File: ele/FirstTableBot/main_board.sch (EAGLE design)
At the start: 2 parts

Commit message: Vzber sensoru
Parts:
- removed JP1: PINH2X06, pinhead_smd:PINH2X06
- added JP2: PINH2X08, pinhead_smd:PINH2X08
- added R1, R10, R11, R12, R13, R14, R2, R3, R4, R5, R6, R7, R8, R9: (no value), resistor:R-EU_R0603
- added U$1, U$2, U$3, U$4, U$5, U$6, U$7: CNY70, cny70:CNY70
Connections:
- new net ADC0: MLF1.PA3/ADC0/T1/SNS, R2.1, U$2.COL
- new net ADC1: MLF1.PA4/ADC1/T0, R4.1, U$1.COL
- new net ADC11: MLF1.ADC11/CLK0/PC2
- new net ADC2: MLF1.PA5/ADC2/OC0B, R6.1, U$3.COL
- new net ADC3: MLF1.PA6/ADC3/OC1B, R8.1, U$4.COL
- new net ADC4: MLF1.PA7/RXD0/ADC4, R10.1, U$5.COL
- new net ADC5: MLF1.PB0/TXD0/ADC5, R12.1, U$6.COL
- new net ADC6: R14.1, U$7.COL
- new net ADC8: MLF1.ADC8/OC1A/PB3
- new net ADC9: MLF1.ADC9/OC0A/XCK0/PC0
- new net N$1: R1.2, U$2.A
- new net N$2: R3.2, U$1.A
- new net N$3: R5.2, U$3.A
- new net N$4: R7.2, U$4.A
- new net N$5: R9.2, U$5.A
- new net N$6: R11.2, U$6.A
- new net N$7: R13.2, U$7.A
- new net SCK: JP2B6.1, JP2T6.1
- net +5V: now also JP2B2.1, JP2T2.1, R1.1, R10.2, R11.1, R12.2, R13.1, R14.2, R2.2, R3.1, R4.2, R5.1, R6.2, R7.1, R8.2, R9.1; no longer JP1B1.1, JP1T1.1
- net CLK: now also JP2B5.1, JP2T5.1; no longer JP1B4.1, JP1T4.1
- net GND: now also JP2B3.1, JP2B4.1, JP2T3.1, JP2T4.1, U$1.C, U$1.EMI, U$2.C, U$2.EMI, U$3.C, U$3.EMI, U$4.C, U$4.EMI, U$5.C, U$5.EMI, U$6.C, U$6.EMI, U$7.C, U$7.EMI; no longer JP1B6.1, JP1T6.1
- net MISO: now also JP2B7.1, JP2T7.1; no longer JP1B3.1, JP1T3.1
- net MOSI: now also JP2B8.1, JP2T8.1; no longer JP1B2.1, JP1T2.1
- net RESET: now also JP2B1.1, JP2T1.1; no longer JP1B5.1, JP1T5.1

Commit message: schem
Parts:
- added C1, C2: 10u, rcl_upravena:C-EUC1206
- added C3, C4, C5, C8, C9: 100n, rcl_upravena:C-EUC1206
- added C6, C7: (no value), rcl:CPOL-EUE5-10.5
- added D2: (no value), diode:DIODE-D-7.5
- added D3: (no value), diode:SCHOTTKY-DIODEF126Z12
- added IM10: DRV8833_BOARD, DRV8833board:DRV8833_BOARD
- added IM6: DEVKITC, esp32:DEVKITC
- added JP3, JP5, JP6: (no value), pinhead:PINHD-1X3
- added JP30: IM10_ULT, pinhead:PINHD-1X1
- added JP4: (no value), pinhead:PINHD-2X5
- added LED0, LED1, LED2, LED3, LED5: BLUE, led:LED3MM
- added LED4: RED, led:LED3MM
- added NC1, NC2, NC3, NC4, NC5, NC6: NC, NC:NC
- added Q2, Q5: (no value), transistors:P-MOSFET-TO220V
- added Q3: (no value), transistors:N-MOSFET-SOT23-DIST
- added Q6: (no value), transistors:N-MOSFET-SOT23-GSD
- added R15: 2M, rcl_upravena:R-EU_R0805
- added R16, R19: 10k, rcl_upravena:R-EU_R0805
- added R17: 100k, rcl_upravena:R-EU_R0805
- added R18: 2M, rcl_upravena:R-EU_M0805
- added R20: (no value), pot:TRIM_US-SM-42/43X
- added R21, R22: 5k, resistor:R-EU_R0402
- added R24: (no value), resistor:R-EU_R0603
- added RN1: (no value), resistor-dil:2R-NEXB24V
- added RN2: (no value), resistor-dil:4R-N0402ARV341
- added SW0, SW1, SW2, SW3, SW4, SW5, SW6: (no value), switch-omron:10-XX
- added X1, X2: M8, con-wago-508:W237-02P
- added X4: POWER_IN, con-wago-508:W237-02P
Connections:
- new net +3V3: IM6.3V3, Q3.G, R16.1, R19.2, R22.1
- new net +5V_ESP: D2.C, IM6.5V
- new net BAT1: Q5.D, X4-2.KL
- new net BAT_POL+: Q2.S, Q5.S, R17.1, R24.2
- new net EN: IM6.EN, R19.1
- new net GPIO0: IM6.IO0
- new net GPIO12: IM6.IO12
- new net GPIO14: IM6.IO14
- new net GPIO15: IM6.IO15
- new net GPIO16: IM6.IO16, JP5.1
- new net GPIO17: IM6.IO17, JP3.1
- new net GPIO18: IM6.IO18
- new net GPIO19: IM6.IO19
- new net GPIO2: IM6.IO2
- new net GPIO21: IM6.IO21, Q3.S, R22.2
- new net GPIO22: IM6.IO22
- new net GPIO23: IM6.IO23
- new net GPIO25: IM6.IO25
- new net GPIO26: IM6.IO26
- new net GPIO27: IM6.IO27
- new net GPIO32: IM6.IO32
- new net GPIO33: IM6.IO33, R20.S
- new net GPIO34: IM6.IO34
- new net GPIO35: IM6.IO35
- new net GPIO36: IM6.SVP
- new net GPIO39: IM6.SVN
- new net GPIO4: IM6.IO4
- new net GPIO5: IM6.IO5
- new net IO1: IM6.TXD0
- new net IO10_NC: IM6.SD3, NC2.NC
- new net IO10_NC1: IM6.SD0, NC5.NC
- new net IO11_NC: IM6.CMD, NC3.NC
- new net IO11_NC1: IM6.SD1, NC6.NC
- new net IO3: IM6.RXD0
- new net IO9_NC: IM6.SD2, NC1.NC
- new net IO9_NC1: IM6.CLK, NC4.NC
- new net M1A: IM10.OUT1, X1-1.KL
- new net M1B: IM10.OUT2, X1-2.KL
- new net M2A: IM10.OUT3, X2-1.KL
- new net M2B: IM10.OUT4, X2-2.KL
- new net N$10: LED5.A, R24.1
- new net N$11: JP6.1, Q3.D, R21.1
- new net N$8: IM10.ULT, JP30.1
- new net N$9: C2.1, Q6.G, R15.1, R16.2, SW5.P, SW5.P1
- new net OFF: IM6.IO13
- new net PA0: MLF1.PA0/AREF, RN2A.1
- new net PA1: MLF1.PA1/AIN0, RN2B.1
- new net PA2: MLF1.PA2/AIN1, RN2C.1
- new net PC4: MLF1.XTAL2/PC4, RN2D.1
- new net PC5: MLF1.XTAL1/PC5, RN1A.1
- new net PWM0: IM10.IN1
- new net PWM1: IM10.IN2
- new net PWM2: IM10.IN3
- new net PWM3: IM10.IN4
- new net SLEEP: IM10.!SLEEP
- new net START_GATE1: C1.1, Q2.G, Q6.D, R17.2, R18.1
- new net SW0: C5.2, JP4.10, LED3.A, RN2A.2, SW0.P, SW0.P1
- new net SW1: C3.2, JP4.8, LED2.A, RN2B.2, SW1.P, SW1.P1
- new net SW2: C4.2, JP4.6, LED1.A, RN2C.2, SW2.P, SW2.P1
- new net SW3: C8.2, JP4.4, LED0.A, RN2D.2, SW3.P, SW3.P1
- new net SW4: C9.2, JP4.2, LED4.A, RN1A.2, SW6.P, SW6.P1
- new net VCC: C6.+, C7.+, D3.C, IM10.VCC, JP3.2, JP5.2, Q2.D, R20.A
- net +5V: now also D2.A, JP6.2, R21.2
- net GND: now also C1.2, C2.2, C3.1, C4.1, C5.1, C6.-, C7.-, C8.1, C9.1, D3.A, IM10.GND, IM6.GND, JP3.3, JP4.1, JP4.3, JP4.5, JP4.7, JP4.9, JP5.3, JP6.3, LED0.C, LED1.C, LED2.C, LED3.C, LED4.C, LED5.C, Q5.G, Q6.S, R15.2, R18.2, R20.E, SW0.S, SW0.S1, SW1.S, SW1.S1, SW2.S, SW2.S1, SW3.S, SW3.S1, SW4.P, SW4.P1, SW4.S, SW4.S1, SW5.S, SW5.S1, SW6.S, SW6.S1, X4-1.KL
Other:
- note added: "delic na mereni baterek"
- note added: "inteligentní ledky"
- note added: "rezerve_ADC1"

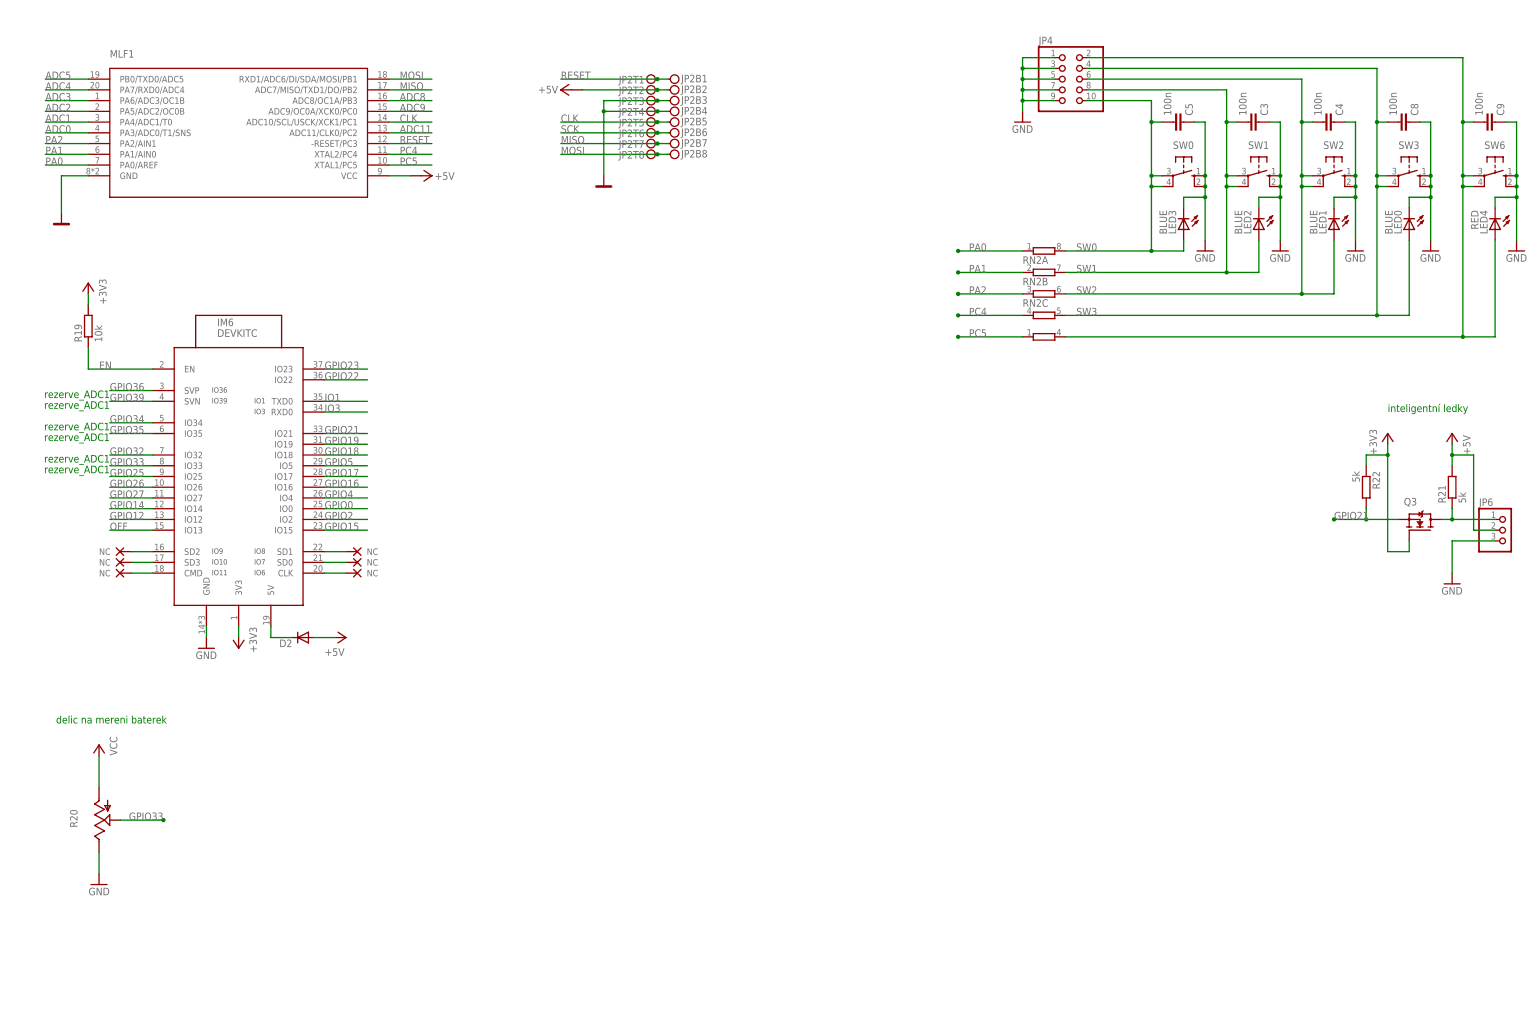
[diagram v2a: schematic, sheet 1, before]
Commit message: zmena ATtiny
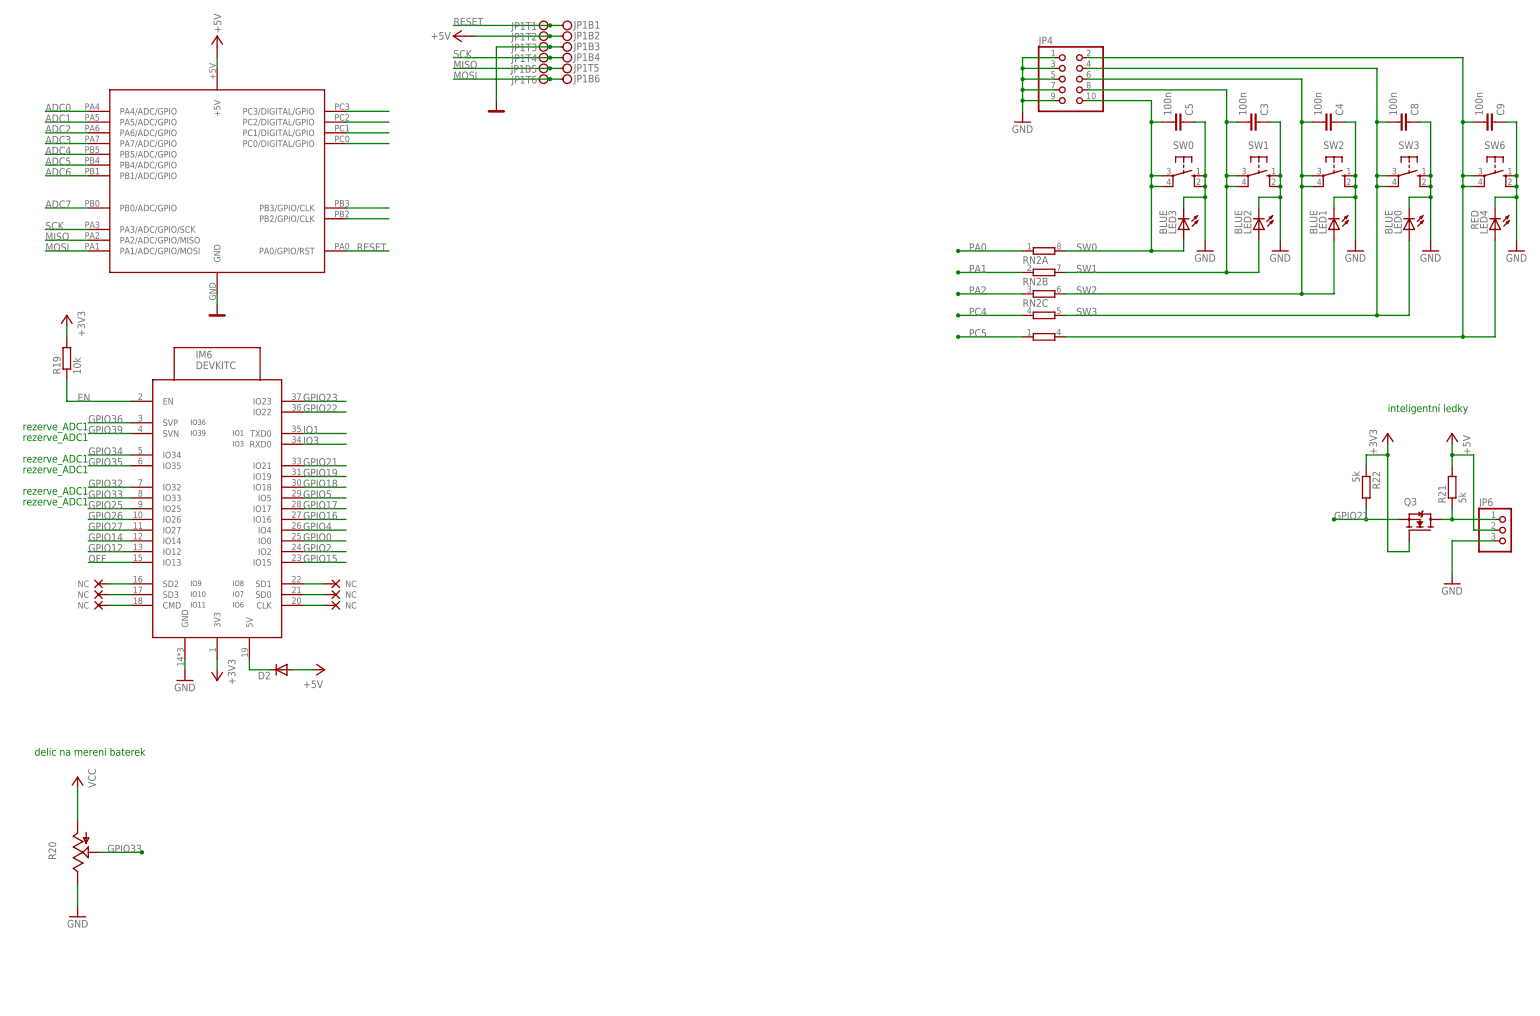
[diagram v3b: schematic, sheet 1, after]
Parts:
- removed JP2: PINH2X08, pinhead_smd:PINH2X08
- removed MLF1: ATTINY1634MLF20, attiny1634:ATTINY1634MLF20
- added JP1: PINH2X06, pinhead_smd:PINH2X06
- added U$8: ATTINI1616SOIC, ATTINY1616:ATTINI1616SOIC
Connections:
- removed net ADC11: MLF1.ADC11/CLK0/PC2
- removed net ADC8: MLF1.ADC8/OC1A/PB3
- removed net ADC9: MLF1.ADC9/OC0A/XCK0/PC0
- removed net CLK: JP2B5.1, JP2T5.1, MLF1.ADC10/SCL/USCK/XCK1/PC1
- new net ADC7: U$8.PB0/ADC/GPIO
- new net N$24: U$8.PB2/GPIO/CLK
- new net N$25: U$8.PB3/GPIO/CLK
- new net N$26: U$8.PC0/DIGITAL/GPIO
- new net N$27: U$8.PC1/DIGITAL/GPIO
- new net N$28: U$8.PC2/DIGITAL/GPIO
- new net N$29: U$8.PC3/DIGITAL/GPIO
- net +5V: now also JP1B2.1, JP1T2.1, U$8.+5V; no longer JP2B2.1, JP2T2.1, MLF1.VCC
- net ADC0: now also U$8.PA4/ADC/GPIO; no longer MLF1.PA3/ADC0/T1/SNS
- net ADC1: now also U$8.PA5/ADC/GPIO; no longer MLF1.PA4/ADC1/T0
- net ADC2: now also U$8.PA6/ADC/GPIO; no longer MLF1.PA5/ADC2/OC0B
- net ADC3: now also U$8.PA7/ADC/GPIO; no longer MLF1.PA6/ADC3/OC1B
- net ADC4: now also U$8.PB5/ADC/GPIO; no longer MLF1.PA7/RXD0/ADC4
- net ADC5: now also U$8.PB4/ADC/GPIO; no longer MLF1.PB0/TXD0/ADC5
- net ADC6: now also U$8.PB1/ADC/GPIO
- net GND: now also JP1B3.1, JP1T3.1, U$8.GND; no longer JP2B3.1, JP2B4.1, JP2T3.1, JP2T4.1, MLF1.GND
- net MISO: now also JP1B5.1, JP1T5.1, U$8.PA2/ADC/GPIO/MISO; no longer JP2B7.1, JP2T7.1, MLF1.ADC7/MISO/TXD1/DO/PB2
- net MOSI: now also JP1B6.1, JP1T6.1, U$8.PA1/ADC/GPIO/MOSI; no longer JP2B8.1, JP2T8.1, MLF1.RXD1/ADC6/DI/SDA/MOSI/PB1
- net PA0: no longer MLF1.PA0/AREF
- net PA1: no longer MLF1.PA1/AIN0
- net PA2: no longer MLF1.PA2/AIN1
- net PC4: no longer MLF1.XTAL2/PC4
- net PC5: no longer MLF1.XTAL1/PC5
- net RESET: now also JP1B1.1, JP1T1.1, U$8.PA0/GPIO/RST; no longer JP2B1.1, JP2T1.1, MLF1.-RESET/PC3
- net SCK: now also JP1B4.1, JP1T4.1, U$8.PA3/ADC/GPIO/SCK; no longer JP2B6.1, JP2T6.1
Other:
- moved on the sheet: D2, IM6, R19, R20

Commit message: DRV8833_jen_svab
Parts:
- removed D2: (no value), diode:DIODE-D-7.5
- removed IM10: DRV8833_BOARD, DRV8833board:DRV8833_BOARD
- removed IM6: DEVKITC, esp32:DEVKITC
- removed JP30: IM10_ULT, pinhead:PINHD-1X1
- removed NC2, NC3, NC4, NC5, NC6: NC, NC:NC
- removed R19: 10k, rcl_upravena:R-EU_R0805
- removed X1, X2: M8, con-wago-508:W237-02P
- added !CTS, !DCD, !DSR, !DTR, !RESET, !RTS, !SUSPEND, CHR0, CHR1, CHREN, IO0/TXLED, IO1/RXLED, IO2/RS485, IO3/WAKEUP, IO4, IO5, IO6, RI/CLK, RXD, SUSPEND, TXD: PINH1X01, pinhead_smd:PINH1X01
- added B1, B2: TACTM-35N-F, TACTM-35N-F:TACTM-35N-F
- added C10, C14, C19, C22: 100n/16V, rcl_upravena:C-EUC0402
- added C11, C12, C13, C18: 4u7/16V, rcl_upravena:C-EUC0603
- added C23: 100nf, resistor:C-EUC0603
- added C37: 330u/16V, rcl_upravena:CPOL-EUE5-10.5
- added D1, D4: skl34, diode:SHOTTKY-SOD123
- added EN, JP36, JP38, VUSB: (no value), pinhead:PINHD-1X2
- added IC3: CP2102N-28, CP2102N:CP2102N-28
- added IM3: STEPDOWN, StepDown:STEPDOWN
- added JP11: (no value), pinhead:PINHD-1X8
- added JP2, PWR_1: (no value), pinhead:PINHD-2X12
- added JP7, PWR_2: (no value), pinhead:PINHD-2X14
- added LED6, LED7, LED8: yellow, led:LEDCHIP-LED0603
- added LED_3V3: green, led:LEDCHIPLED_0603
- added NC7: NC, NC:NC
- added R23, R25, R26, R31: 470R, rcl_upravena:R-EU_R0603
- added R27, R28, R58, R60, R61: 10k, rcl_upravena:R-EU_R0603
- added R29, R30, R32, R33, R34, R35, R36, R37, R38, R39, R40, R41, R42, R43, R44, R45, R46, R47, R48, R49, R50, R51, R52, R53, R54, R55, R56, R57: 180R, rcl_upravena:R-EU_R0603
- added R59: 100k, rcl_upravena:R-EU_R0603
- added T1, T2: BC337, transistors:NPN-SOT23-BEC
- added U$9: DRV8833HTSSOP, texas-cc2541:DRV8833HTSSOP
- added U1: ESP-WROOM-32, esp32:ESP-WROOM-32
- added U2: UM18533, um185xx:UM185XX
- added USB: (no value), pinhead:PINHD-1X5
- added VCC, VCCIO: (no value), pinhead:PINHD-2X3
- added X3: USB-MICRO-B-BOTTOM, usb:USB-MICRO-B-BOTTOM
- C7: value (none) -> 2,2uf; device rcl:CPOL-EUE5-10.5 -> resistor:C-EUC0805
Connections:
- removed net +5V_ESP: D2.C, IM6.5V
- removed net GPIO0: IM6.IO0
- removed net GPIO12: IM6.IO12
- removed net GPIO14: IM6.IO14
- removed net GPIO15: IM6.IO15
- removed net GPIO18: IM6.IO18
- removed net GPIO19: IM6.IO19
- removed net GPIO2: IM6.IO2
- removed net GPIO22: IM6.IO22
- removed net GPIO23: IM6.IO23
- removed net GPIO25: IM6.IO25
- removed net GPIO26: IM6.IO26
- removed net GPIO27: IM6.IO27
- removed net GPIO32: IM6.IO32
- removed net GPIO34: IM6.IO34
- removed net GPIO35: IM6.IO35
- removed net GPIO36: IM6.SVP
- removed net GPIO39: IM6.SVN
- removed net GPIO4: IM6.IO4
- removed net GPIO5: IM6.IO5
- removed net IO1: IM6.TXD0
- removed net IO10_NC: IM6.SD3, NC2.NC
- removed net IO10_NC1: IM6.SD0, NC5.NC
- removed net IO11_NC: IM6.CMD, NC3.NC
- removed net IO11_NC1: IM6.SD1, NC6.NC
- removed net IO3: IM6.RXD0
- removed net IO9_NC: IM6.SD2, NC1.NC
- removed net IO9_NC1: IM6.CLK, NC4.NC
- removed net M1A: IM10.OUT1, X1-1.KL
- removed net M1B: IM10.OUT2, X1-2.KL
- removed net M2A: IM10.OUT3, X2-1.KL
- removed net M2B: IM10.OUT4, X2-2.KL
- removed net N$26: U$8.PC0/DIGITAL/GPIO
- removed net N$27: U$8.PC1/DIGITAL/GPIO
- removed net N$28: U$8.PC2/DIGITAL/GPIO
- removed net N$29: U$8.PC3/DIGITAL/GPIO
- removed net OFF: IM6.IO13
- removed net PA0: RN2A.1
- removed net PA1: RN2B.1
- removed net PA2: RN2C.1
- removed net PC4: RN2D.1
- removed net PC5: RN1A.1
- removed net PWM0: IM10.IN1
- removed net PWM1: IM10.IN2
- removed net PWM2: IM10.IN3
- removed net PWM3: IM10.IN4
- new net !DTR: !DTR.1, IC3.!DTR, R27.1, T2.E
- new net !DTR_B: R27.2, T1.B
- new net !RESET: !RESET.1, IC3.!RESET, R58.1
- new net !RTS: !RTS.1, IC3.!RTS, R28.1, T1.E
- new net !RTS_B: R28.2, T2.B
- new net !SHDN: JP36.2, R59.2, U2.!SHDN
- new net !SUSPEND: !SUSPEND.1, IC3.!SUSPEND
- new net 3V3_IN: C12.1, C37.+, D1.C, R59.1, U2.IN
- new net 5V_USB: D4.C, VUSB.1
- new net BTN0: B1.P$4, C19.2, JP38.1, R61.1
- new net BTN1: B2.P$4, C22.2, JP38.2, R60.1
- new net CHR0: CHR0.1, IC3.CHR0
- new net CHR1: CHR1.1, IC3.CHR1
- new net CHREN: CHREN.1, IC3.CHREN
- new net CLK/!RI: IC3.CLK/!RI, RI/CLK.1
- new net DCD: !DCD.1, IC3.!DCD
- new net DM: IC3.USBDM, USB.2, X3.D-
- new net DP: IC3.USBDP, USB.3, X3.D+
- new net DSR: !DSR.1, IC3.!DSR
- new net IO0_!RST: JP7.23, R52.1
- new net IO0_!RST!_: R52.2, T2.C, U1.IO0
- new net IO12: JP2.22, R41.1
- new net IO12_: R41.2, U1.IO12
- new net IO13: JP2.24, R42.1
- new net IO13_: R42.2, U1.IO13
- new net IO14: JP2.20, R40.1
- new net IO14_: R40.2, U1.IO14
- new net IO15: JP7.27, R56.1
- new net IO15_: R56.2, U1.IO15
- new net IO16: JP7.19, R50.1
- new net IO16_: R50.2, U1.IO16
- new net IO17: JP7.17, R49.1
- new net IO17_: R49.2, U1.IO17
- new net IO18: JP7.13, R47.1
- new net IO18_: R47.2, U1.IO18
- new net IO19: JP7.11, R46.1
- new net IO19_: R46.2, U1.IO19
- new net IO2: JP7.25, R53.1
- new net IO21: JP7.9, R45.1
- new net IO21_: R45.2, U1.IO21
- new net IO22: JP7.3, R43.1
- new net IO22_: R43.2, U1.IO22
- new net IO23: JP7.1, R54.1
- new net IO23_: R54.2, U1.IO23
- new net IO25: JP2.14, R37.1
- new net IO25_: R37.2, U1.IO25
- new net IO26: JP2.16, R38.1
- new net IO26_: R38.2, U1.IO26
- new net IO27: JP2.18, R39.1
- new net IO27_: R39.2, U1.IO27
- new net IO2_: R53.2, U1.IO2
- new net IO32: JP2.10, R35.1
- new net IO32_: R35.2, U1.IO32
- new net IO33: JP2.12, R36.1
- new net IO33_: R36.2, U1.IO33
- new net IO34: JP2.6, R33.1
- new net IO34_: R33.2, U1.IO34
- new net IO35: JP2.8, R34.1
- new net IO35_: R34.2, U1.IO35
- new net IO4: JP7.21, R51.1
- new net IO4_: R51.2, U1.IO4
- new net IO5: JP7.15, R48.1
- new net IO5_: R48.2, U1.IO5
- new net IO9_NC2: IM3.EN, NC1.NC
- new net LED_3V3: LED_3V3.C, R31.2
- new net N$12: !CTS.1, IC3.!CTS
- new net N$13: LED8.C, R26.2
- new net N$14: U$9.AUOT2
- new net N$15: U$9.BOUT1
- new net N$16: U$9.BOUT2
- new net N$17: U$9.NFAULT
- new net N$23: C7.1, U$9.VINT
- new net NC-CS: JP11.3, U1.CMD
- new net NC-HOLD: JP11.1, U1.SD2
- new net NC-MISO: JP11.6, U1.SD1
- new net NC-MOSI: JP11.5, U1.SD0
- new net NC-SCK: JP11.4, U1.CLK
- new net NC-WP: JP11.2, U1.SD3
- new net PB3: RN1A.1, U$8.PB3/GPIO/CLK
- new net PC0: RN2A.1, U$8.PC0/DIGITAL/GPIO
- new net PC1: RN2B.1, U$8.PC1/DIGITAL/GPIO
- new net PC2: RN2C.1, U$8.PC2/DIGITAL/GPIO
- new net PC3: RN2D.1, U$8.PC3/DIGITAL/GPIO
- new net PWM_A1: U$9.AIN1
- new net PWM_A2: U$9.AIN2
- new net PWM_B1: U$9.BIN1
- new net PWM_B2: U$9.BIN2
- new net RX-LED: LED7.C, R25.1
- new net RXD: IC3.RXD, R30.1, RXD.1
- new net RXD0: JP7.7, R55.1
- new net RXD0_: R29.2, R55.2, U1.RXD0
- new net RX_LED: IC3.RXLED/IO1, IO1/RXLED.1, R25.2
- new net SENSOR_VN: JP2.4, R32.1
- new net SENSOR_VN_: R32.2, U1.SENSOR_VN
- new net SENSOR_VP: JP2.2, R57.1
- new net SENSOR_VP_: R57.2, U1.SENSOR_VP
- new net SUSPEND: IC3.SUSPEND, R26.1, SUSPEND.1
- new net TX-LED: LED6.C, R23.1
- new net TXD: IC3.TXD, R29.1, TXD.1
- new net TXD0: JP7.5, R44.1
- new net TXD0_: R30.2, R44.2, U1.TXD0
- new net TX_LED: IC3.TXLED/IO0, IO0/TXLED.1, R23.2
- new net U2_NC: NC7.NC, U2.NC
- new net USBID: USB.4, X3.ID
- new net USBIO3_RS485: IC3.RS485/IO2, IO2/RS485.1
- new net USBIO3_WAKEUP: IC3.WAKEUP/IO3, IO3/WAKEUP.1
- new net USBIO4: IC3.IO4, IO4.1
- new net USBIO5: IC3.IO5, IO5.1
- new net USBIO6: IC3.IO6, IO6.1
- new net VCCIO: C10.1, C18.1, IC3.VCC, LED6.A, LED7.A, LED8.A, R58.2, VCCIO.2, VCCIO.4, VCCIO.6
- new net VUSB: C11.1, C14.1, D4.A, IC3.VBUS, IC3.VREGIN, USB.1, X3.VBUS
- net +3V3: now also C13.1, JP11.8, LED_3V3.A, PWR_1.10, PWR_1.12, PWR_1.14, PWR_1.16, PWR_1.18, PWR_1.2, PWR_1.20, PWR_1.22, PWR_1.24, PWR_1.4, PWR_1.6, PWR_1.8, PWR_2.10, PWR_2.12, PWR_2.14, PWR_2.16, PWR_2.18, PWR_2.2, PWR_2.20, PWR_2.22, PWR_2.24, PWR_2.26, PWR_2.28, PWR_2.4, PWR_2.6, PWR_2.8, R60.2, R61.2, U1.3V3, U2.OUT; no longer IM6.3V3, R19.2
- net +5V: now also D1.A, IM3.OUT, PWR_1.1, PWR_1.11, PWR_1.13, PWR_1.15, PWR_1.17, PWR_1.19, PWR_1.21, PWR_1.23, PWR_1.3, PWR_1.5, PWR_1.7, PWR_1.9, PWR_2.1, PWR_2.11, PWR_2.13, PWR_2.15, PWR_2.17, PWR_2.19, PWR_2.21, PWR_2.23, PWR_2.25, PWR_2.27, PWR_2.3, PWR_2.5, PWR_2.7, PWR_2.9, VUSB.2; no longer D2.A
- net EN: now also EN.1, T1.C, U1.EN; no longer IM6.EN, R19.1
- net GND: now also B1.P$3, B2.P$3, C10.2, C11.2, C12.2, C13.2, C14.2, C18.2, C19.1, C22.1, C37.-, C7.2, EN.2, IC3.GND, IM3.GND, JP11.7, JP2.1, JP2.11, JP2.13, JP2.15, JP2.17, JP2.19, JP2.21, JP2.23, JP2.3, JP2.5, JP2.7, JP2.9, JP36.1, JP7.10, JP7.12, JP7.14, JP7.16, JP7.18, JP7.2, JP7.20, JP7.22, JP7.24, JP7.26, JP7.28, JP7.4, JP7.6, JP7.8, R31.1, U$9.AISEN, U$9.BISEN, U$9.GND, U1.GND@1, U1.GND@2, U1.GND@3, U1.GND@4, U2.GND, USB.5, VCC.1, VCC.3, VCC.5, VCCIO.1, VCCIO.3, VCCIO.5, X3.GND; no longer C7.-, IM10.GND, IM6.GND
- net GPIO16: no longer IM6.IO16
- net GPIO17: no longer IM6.IO17
- net GPIO21: no longer IM6.IO21
- net GPIO33: no longer IM6.IO33
- net N$25: now also C23.1, U$9.VCP; no longer U$8.PB3/GPIO/CLK
- net N$8: now also U$9.AOUT1; no longer IM10.ULT, JP30.1
- net SLEEP: now also U$9.NSLEEP; no longer IM10.!SLEEP
- net VCC: now also C23.2, IM3.IN, U$9.VM_2.7-10.8V, VCC.2, VCC.4, VCC.6; no longer C7.+, IM10.VCC
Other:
- note added: "RobotikaBrno"
- note added: "github:roboticsbrno/ RB3200-ESP32universal RobotikaBrno.cz Robotarna CC BY-SA 4.0"
- note added: "v2.0"
- note removed: "rezerve_ADC1"
